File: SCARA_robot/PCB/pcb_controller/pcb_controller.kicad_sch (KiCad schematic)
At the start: 41 parts, among them IC1 LD1117-3.3V-SOT223, J1 Barrel_Jack_Switch, J10 interface, J11 Conn_01x07_Socket, J12 Encoder_A, J13 Encoder_B, J14 Encoder_C, J2 Conn_01x04_Pin_STEPPER_A, J3 interface, J4 power, J5 Conn_01x07_Socket, J6 power, J7 interface, J8 Conn_01x07_Socket, J9 power, SW1 Microstep mode, U1 LM7805CT, U2 ESP32-DEVKIT-V1

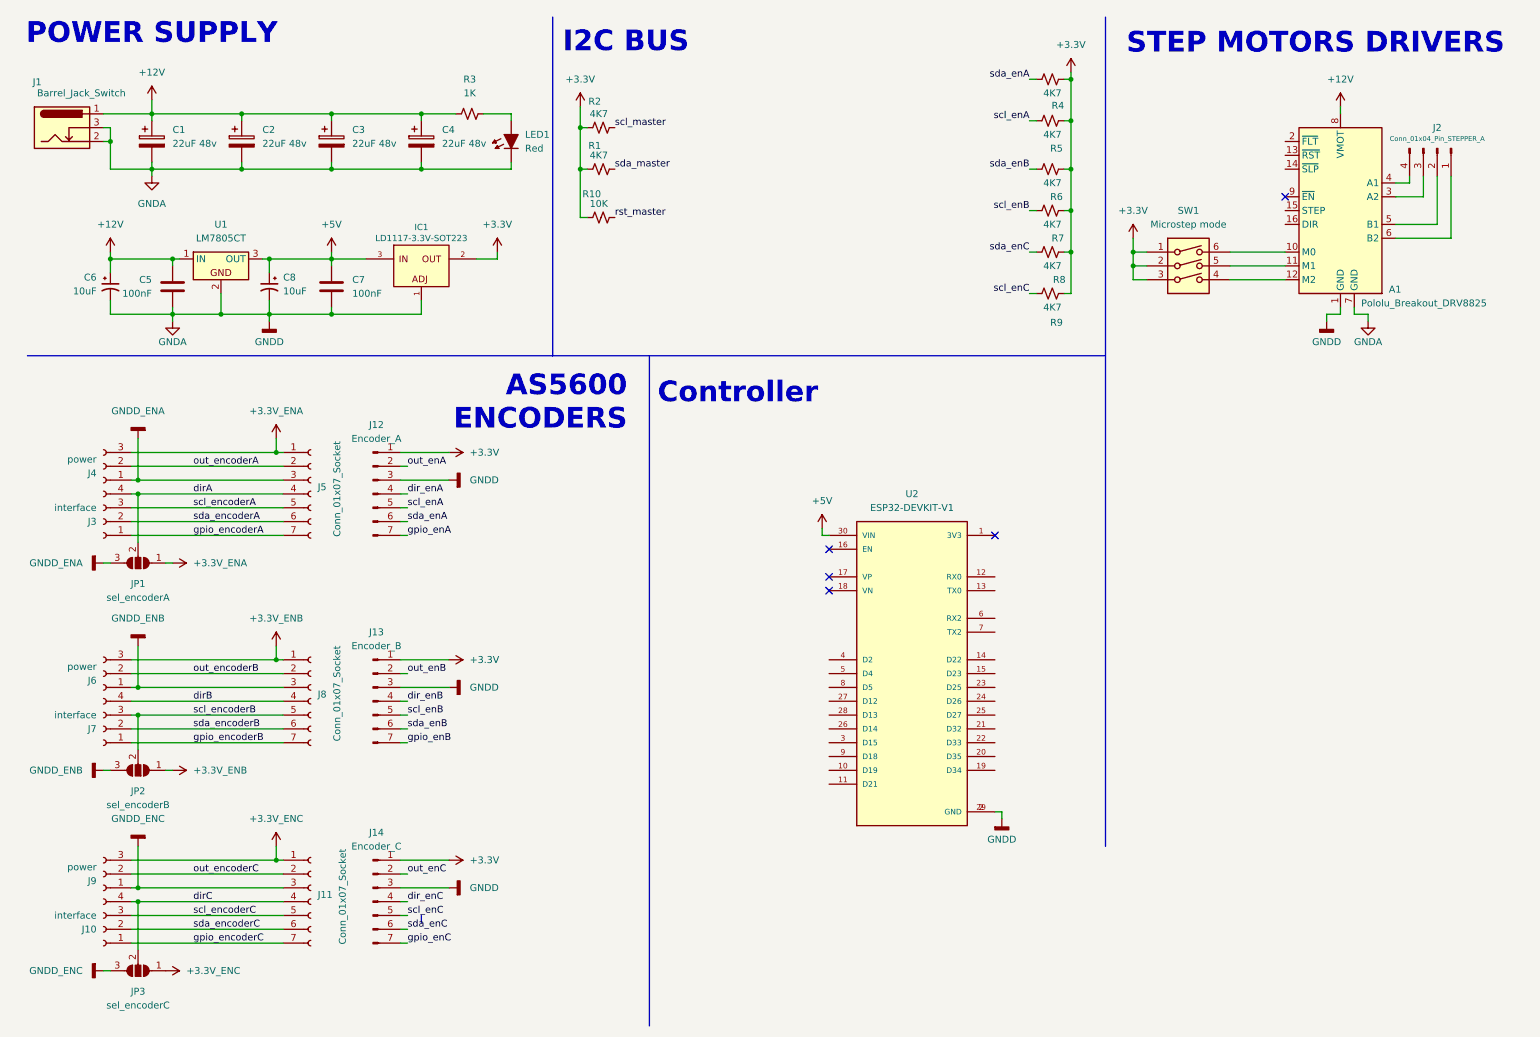
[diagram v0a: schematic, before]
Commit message: schematic ready
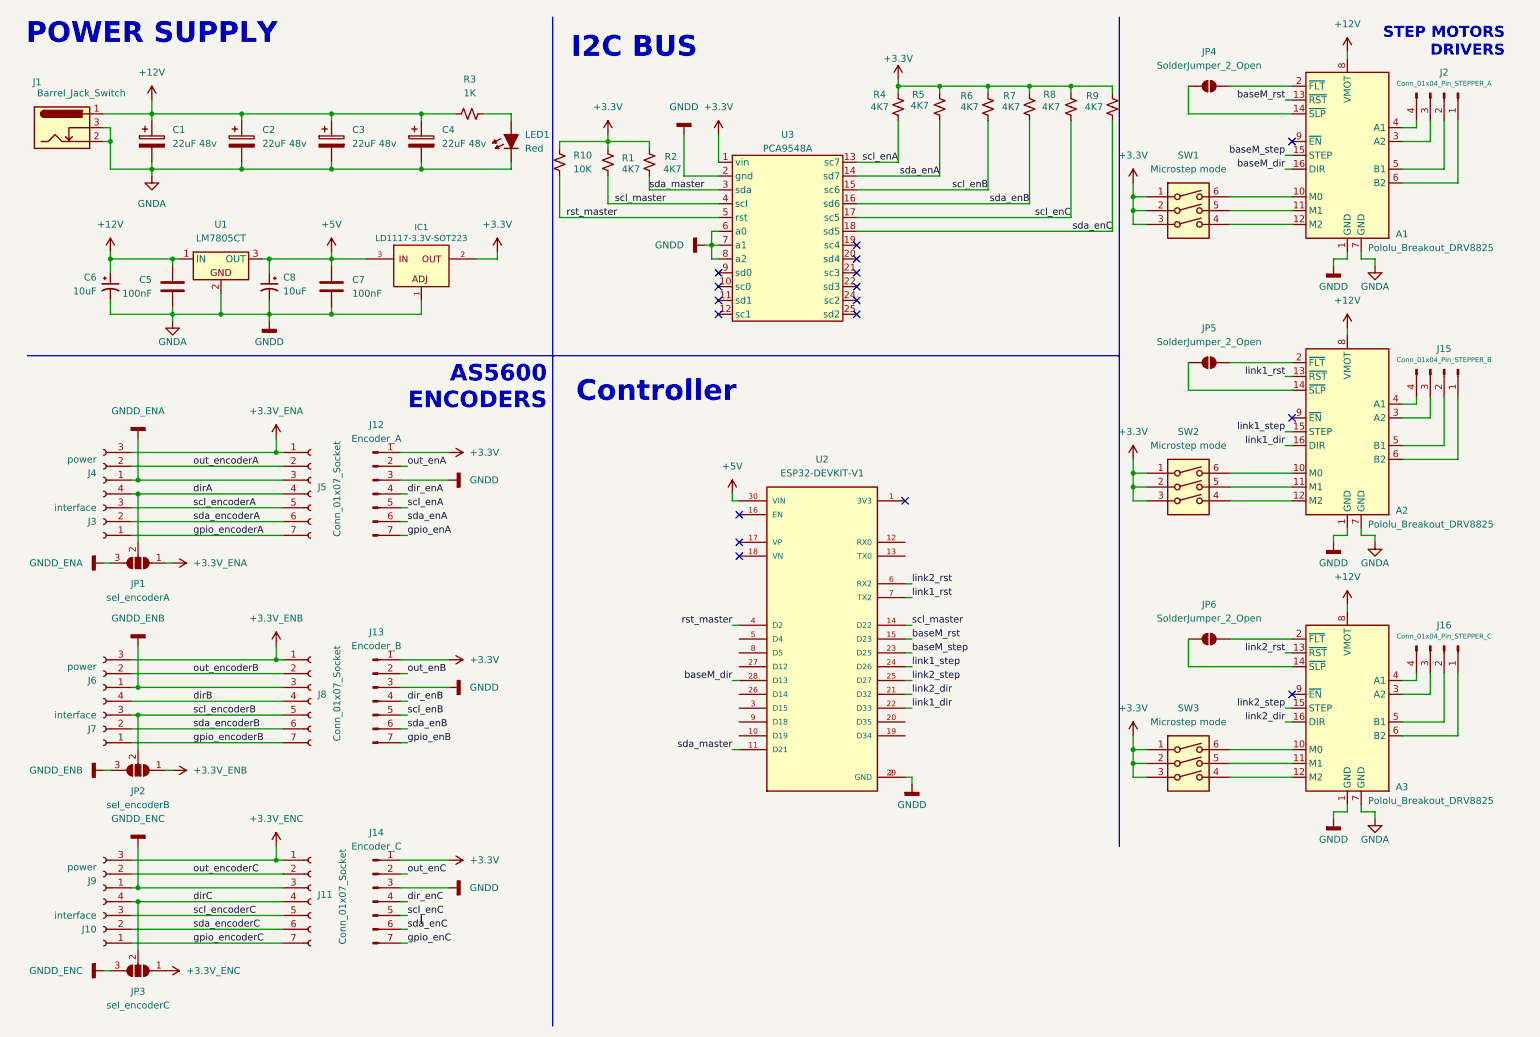
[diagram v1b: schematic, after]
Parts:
- added A2, A3: Pololu_Breakout_DRV8825, Module:Pololu_Breakout-16_15.2x20.3mm, symbol Driver_Motor:Pololu_Breakout_DRV8825
- added J15: Conn_01x04_Pin_STEPPER_B, Connector_JST:JST_XH_B4B-XH-AM_1x04_P2.50mm_Vertical, symbol Connector:Conn_01x04_Pin
- added J16: Conn_01x04_Pin_STEPPER_C, Connector_JST:JST_XH_B4B-XH-AM_1x04_P2.50mm_Vertical, symbol Connector:Conn_01x04_Pin
- added JP4, JP5, JP6: SolderJumper_2_Open, Jumper:SolderJumper-2_P1.3mm_Open_RoundedPad1.0x1.5mm, symbol Jumper:SolderJumper_2_Open
- added SW2, SW3: Microstep mode, Button_Switch_THT:SW_DIP_SPSTx03_Slide_9.78x9.8mm_W7.62mm_P2.54mm, symbol Switch:SW_DIP_x03
- added U3: PCA9548A, symbol modules:1{colon}8_i2c_mux
- JP1, JP2, JP3: footprint (none) -> Jumper:SolderJumper-3_P1.3mm_Open_RoundedPad1.0x1.5mm
- SW1: footprint (none) -> Button_Switch_THT:SW_DIP_SPSTx03_Slide_9.78x9.8mm_W7.62mm_P2.54mm
- U1: footprint PCM_Package_TO_SOT_THT_AKL:TO-220-3_Vertical -> PCM_4ms_Package_TO:TO-220-3_Horizontal
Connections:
- net +12V: now also A2.8 (VMOT), A3.8 (VMOT)
- net +3.3V: now also SW2.1, SW2.2, SW2.3, SW3.1, SW3.2, SW3.3, U3.1 (vin)
- net GNDA: now also A2.1 (GND), A2.7 (GND), A3.1 (GND), A3.7 (GND), U3.2 (gnd), U3.6 (a0), U3.7 (a1), U3.8 (a2)
- net rst_master: now also U2.4 (D2), U3.5 (rst)
- net scl_enA: now also R4.2, U3.13 (sc7); no longer R5.2
- net scl_enB: now also R6.2, U3.15 (sc6); no longer R7.2
- net scl_enC: now also R8.2, U3.17 (sc5); no longer R9.2
- net scl_master: now also R1.2, U2.14 (D22), U3.4 (scl); no longer R2.2
- net sda_enA: now also R5.2, U3.14 (sd7); no longer R4.2
- net sda_enB: now also R7.2, U3.16 (sd6); no longer R6.2
- net sda_enC: now also R9.2, U3.18 (sd5); no longer R8.2
- net sda_master: now also R2.2, U2.11 (D21), U3.3 (sda); no longer R1.2
- net baseM_rst: now reaches U2.15 (D23)
- net baseM_rst: now also A1.13 (~{RST})
- net link2_dir: now reaches U2.21 (D32)
- net link2_dir: now also A3.16 (DIR)
- net link1_dir: now reaches U2.22 (D33)
- net link1_dir: now also A2.16 (DIR)
- net baseM_step: now reaches U2.23 (D25)
- net baseM_step: now also A1.15 (STEP)
- net link1_step: now reaches U2.24 (D26)
- net link1_step: now also A2.15 (STEP)
- net link2_step: now reaches U2.25 (D27)
- net link2_step: now also A3.15 (STEP)
- net baseM_dir: now reaches U2.28 (D13)
- net baseM_dir: now also A1.16 (DIR)
- net link2_rst: now reaches U2.6 (RX2)
- net link2_rst: now also A3.13 (~{RST})
- net link1_rst: now reaches U2.7 (TX2)
- net link1_rst: now also A2.13 (~{RST})
- net at A1.14 (~{SLP}): now also JP4.2 (B)
- net at A1.2 (~{FLT}): now also JP4.1 (A)
- new net: A3.12 (M2), SW3.4
- new net: A3.11 (M1), SW3.5
- new net: A3.10 (M0), SW3.6
- new net: A2.12 (M2), SW2.4
- new net: A2.11 (M1), SW2.5
- new net: A2.10 (M0), SW2.6
- new net: A2.6 (B2), J15.1 (Pin_1)
- new net: A2.5 (B1), J15.2 (Pin_2)
- new net: A2.3 (A2), J15.3 (Pin_3)
- new net: A2.4 (A1), J15.4 (Pin_4)
- new net: A2.2 (~{FLT}), JP5.1 (A)
- new net: A2.14 (~{SLP}), JP5.2 (B)
- new net: A3.2 (~{FLT}), JP6.1 (A)
- new net: A3.14 (~{SLP}), JP6.2 (B)
- new net: A3.6 (B2), J16.1 (Pin_1)
- new net: A3.5 (B1), J16.2 (Pin_2)
- new net: A3.3 (A2), J16.3 (Pin_3)
- new net: A3.4 (A1), J16.4 (Pin_4)
- no-connect marks 5 -> 17
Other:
- moved on the sheet: A1, J2, R1, R10, R2, R4, R5, R6, R7, R8, R9, SW1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
